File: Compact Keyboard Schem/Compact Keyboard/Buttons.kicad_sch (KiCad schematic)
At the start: 12 parts, among them SW2 SW_Push, SW3 SW_Push, SW4 SW_Push, SW5 SW_Push

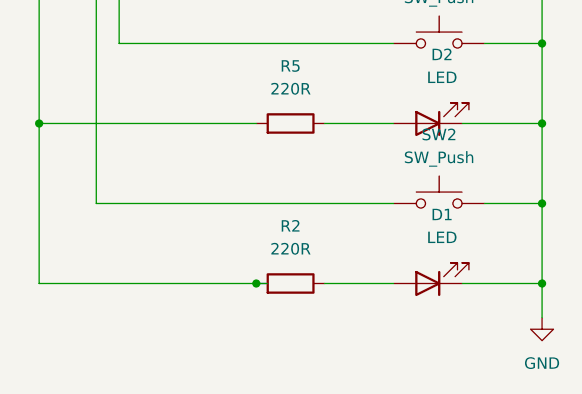
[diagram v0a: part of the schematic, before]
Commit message: Pushing Update
Latest version after PCB printing
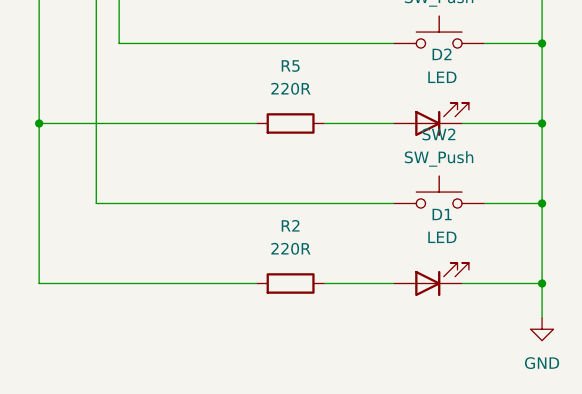
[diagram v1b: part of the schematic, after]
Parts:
- D1, D2, D3, D4: footprint LED_SMD:LED_0402_1005Metric_Pad0.77x0.64mm_HandSolder -> LED_SMD:LED_0805_2012Metric_Pad1.15x1.40mm_HandSolder
- R2, R3, R4, R5: footprint Resistor_THT:R_Axial_DIN0204_L3.6mm_D1.6mm_P7.62mm_Horizontal -> Resistor_SMD:R_0805_2012Metric_Pad1.20x1.40mm_HandSolder
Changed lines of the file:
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@@
-	)
-	(junction
-		(at 135.89 142.24)
-		(diameter 0)
-		(color 0 0 0 0)
 	)
 	(junction
@@
 	(wire
 		(pts
-			(xy 135.89 142.24) (xy 137.16 142.24)
-		)
-		(stroke
-			(width 0)
-			(type default)
-		)
-	)
-	(wire
-		(pts
 			(xy 167.64 124.46) (xy 167.64 133.35)
 		)
@@
 	(wire
 		(pts
+			(xy 143.51 124.46) (xy 151.13 124.46)
+		)
+		(stroke
+			(width 0)
+			(type default)
+		)
+	)
+	(wire
+		(pts
+			(xy 111.76 88.9) (xy 135.89 88.9)
+		)
+		(stroke
+			(width 0)
+			(type default)
+		)
+	)
+	(wire
+		(pts
+			(xy 167.64 142.24) (xy 167.64 146.05)
+		)
+		(stroke
+			(width 0)
+			(type default)
+		)
+	)
+	(wire
+		(pts
+			(xy 120.65 115.57) (xy 151.13 115.57)
+		)
+		(stroke
+			(width 0)
+			(type default)
+		)
+	)
+	(wire
+		(pts
+			(xy 158.75 124.46) (xy 167.64 124.46)
+		)
+		(stroke
+			(width 0)
+			(type default)
+		)
+	)
+	(wire
+		(pts
+			(xy 167.64 115.57) (xy 167.64 124.46)
+		)
+		(stroke
+			(width 0)
+			(type default)
+		)
+	)
+	(wire
+		(pts
 			(xy 111.76 142.24) (xy 135.89 142.24)
-		)
-		(stroke
-			(width 0)
-			(type default)
-		)
-	)
-	(wire
-		(pts
-			(xy 143.51 124.46) (xy 151.13 124.46)
-		)
-		(stroke
-			(width 0)
-			(type default)
-		)
-	)
-	(wire
-		(pts
-			(xy 111.76 88.9) (xy 135.89 88.9)
-		)
-		(stroke
-			(width 0)
-			(type default)
-		)
-	)
-	(wire
-		(pts
-			(xy 167.64 142.24) (xy 167.64 146.05)
-		)
-		(stroke
-			(width 0)
-			(type default)
-		)
-	)
-	(wire
-		(pts
-			(xy 120.65 115.57) (xy 151.13 115.57)
-		)
-		(stroke
-			(width 0)
-			(type default)
-		)
-	)
-	(wire
-		(pts
-			(xy 158.75 124.46) (xy 167.64 124.46)
-		)
-		(stroke
-			(width 0)
-			(type default)
-		)
-	)
-	(wire
-		(pts
-			(xy 167.64 115.57) (xy 167.64 124.46)
 		)
 		(stroke
@@
 			)
 		)
-		(property "Footprint" "Resistor_THT:R_Axial_DIN0204_L3.6mm_D1.6mm_P7.62mm_Horizontal"
+		(property "Footprint" "Resistor_SMD:R_0805_2012Metric_Pad1.20x1.40mm_HandSolder"
 			(at 139.7 126.238 90)
 			(effects
@@
 			)
 		)
-		(property "Footprint" "LED_SMD:LED_0402_1005Metric_Pad0.77x0.64mm_HandSolder"
+		(property "Footprint" "LED_SMD:LED_0805_2012Metric_Pad1.15x1.40mm_HandSolder"
 			(at 154.94 106.68 0)
 			(effects
@@
 			)
 		)
-		(property "Footprint" "Resistor_THT:R_Axial_DIN0204_L3.6mm_D1.6mm_P7.62mm_Horizontal"
+		(property "Footprint" "Resistor_SMD:R_0805_2012Metric_Pad1.20x1.40mm_HandSolder"
 			(at 139.7 144.018 90)
 			(effects
@@
 			)
 		)
-		(property "Footprint" "Resistor_THT:R_Axial_DIN0204_L3.6mm_D1.6mm_P7.62mm_Horizontal"
+		(property "Footprint" "Resistor_SMD:R_0805_2012Metric_Pad1.20x1.40mm_HandSolder"
 			(at 139.7 90.678 90)
 			(effects
@@
 			)
 		)
-		(property "Footprint" "Resistor_THT:R_Axial_DIN0204_L3.6mm_D1.6mm_P7.62mm_Horizontal"
+		(property "Footprint" "Resistor_SMD:R_0805_2012Metric_Pad1.20x1.40mm_HandSolder"
 			(at 139.7 108.458 90)
 			(effects
@@
 			)
 		)
-		(property "Footprint" "LED_SMD:LED_0402_1005Metric_Pad0.77x0.64mm_HandSolder"
+		(property "Footprint" "LED_SMD:LED_0805_2012Metric_Pad1.15x1.40mm_HandSolder"
 			(at 154.94 88.9 0)
 			(effects
@@
 			)
 		)
-		(property "Footprint" "LED_SMD:LED_0402_1005Metric_Pad0.77x0.64mm_HandSolder"
+		(property "Footprint" "LED_SMD:LED_0805_2012Metric_Pad1.15x1.40mm_HandSolder"
 			(at 154.94 142.24 0)
 			(effects
@@
 			)
 		)
-		(property "Footprint" "LED_SMD:LED_0402_1005Metric_Pad0.77x0.64mm_HandSolder"
+		(property "Footprint" "LED_SMD:LED_0805_2012Metric_Pad1.15x1.40mm_HandSolder"
 			(at 154.94 124.46 0)
 			(effects
